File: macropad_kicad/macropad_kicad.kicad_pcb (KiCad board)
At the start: 2 copper layers, 26 parts, among them J1 OLED_128x64, SW1 RotaryEncoder_Switch, U1 MOUDLE-SEEEDUINO-XIAO

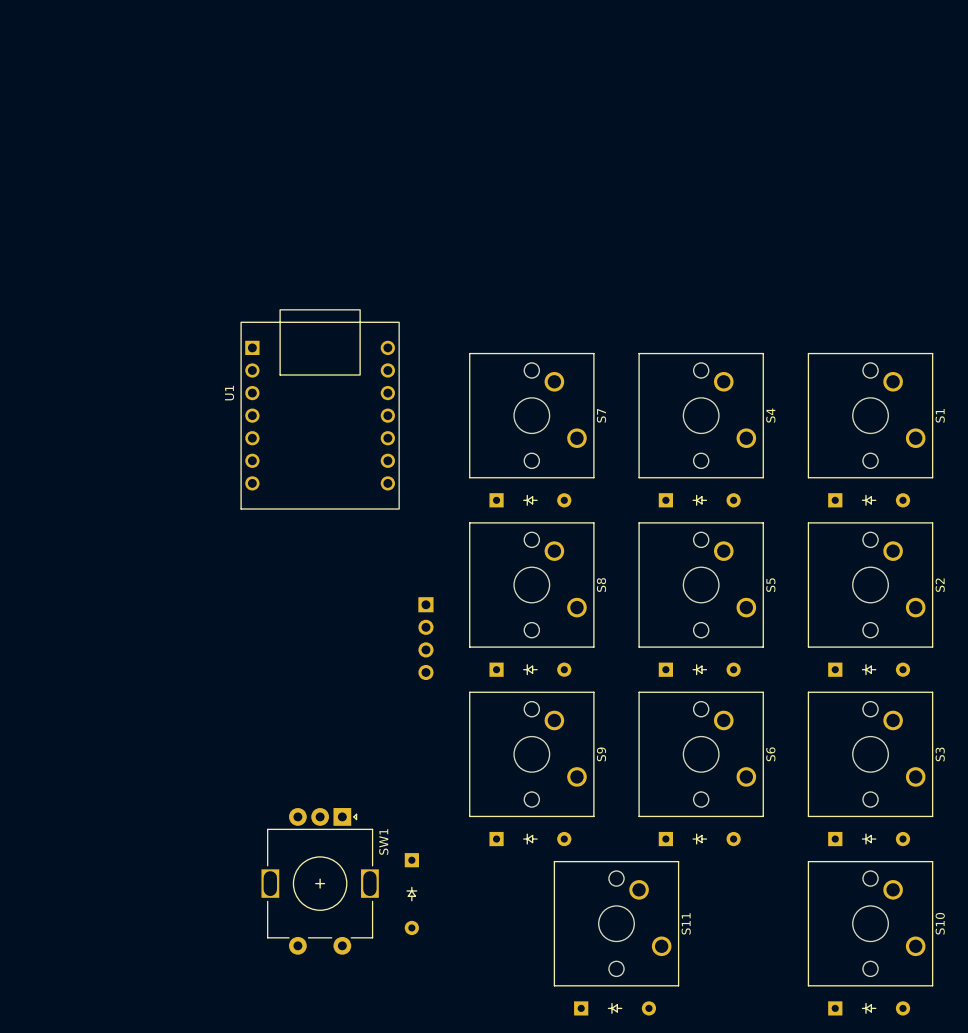
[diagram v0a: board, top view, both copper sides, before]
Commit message: fixed scheme
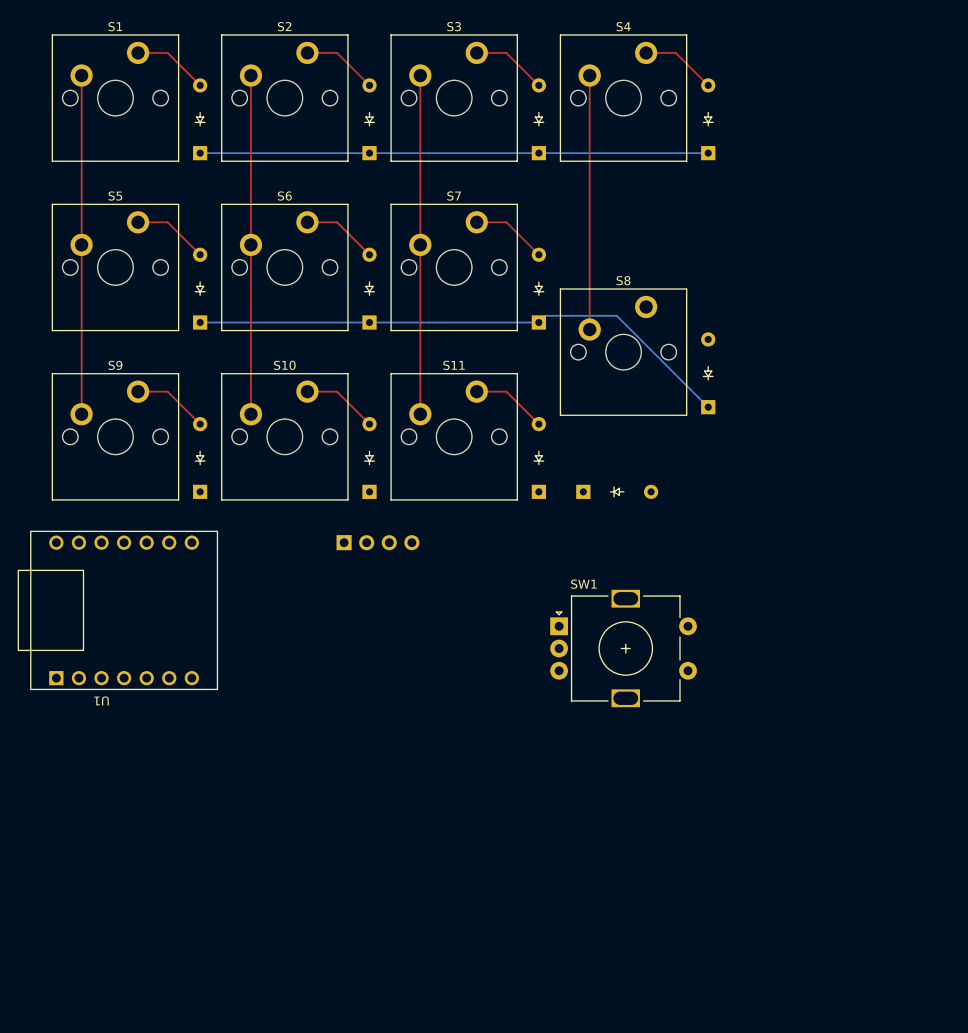
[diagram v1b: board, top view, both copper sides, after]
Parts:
- S1, S10, S11, S2, S3, S4, S5, S6, S7, S8, S9: footprint Button_Switch_Keyboard:SW_Cherry_MX_1.00u_PCB -> ScottoKeebs_MX:MX_PCB_1.00u
- moved S1 97.8 mm to (57.1, 38.1), turned to 0 degrees
- moved S3 92.3 mm to (95.2, 38.1), turned to 0 degrees
- moved S10 91.2 mm to (76.2, 76.2), turned to 0 degrees
- moved S2 91.2 mm to (76.2, 38.1), turned to 0 degrees
- moved D7 84.0 mm to (104.8, 63.3), turned to 90 degrees
- moved S5 80.6 mm to (57.1, 57.1), turned to 0 degrees
- moved D4 78.5 mm to (123.8, 44.3), turned to 90 degrees
- moved D5 78.2 mm to (66.7, 63.3), turned to 90 degrees
- moved S6 77.3 mm to (76.2, 57.1), turned to 0 degrees
- moved D8 69.1 mm to (123.8, 72.9), turned to 90 degrees
- moved D2 67.0 mm to (85.7, 44.3), turned to 90 degrees
- moved D3 67.0 mm to (104.8, 44.3), turned to 90 degrees
- moved D1 65.3 mm to (66.7, 44.3), turned to 90 degrees
- moved S9 64.5 mm to (57.1, 76.2), turned to 0 degrees
- moved S11 61.9 mm to (95.2, 76.2), turned to 0 degrees
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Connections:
- D1 pad 1: (no net) -> Row 0
- D1 pad 2: (no net) -> Net-(D1-A)
- D10 pad 1: Row 0 -> Row 2
- D10 pad 2: (no net) -> Net-(D10-A)
- D11 pad 1: Row 1 -> Row 2
- D11 pad 2: (no net) -> Net-(D11-A)
- D12 pad 2: (no net) -> Net-(D12-A)
- D2 pad 2: (no net) -> Net-(D2-A)
- D3 pad 2: (no net) -> Net-(D3-A)
- D4 pad 1: (no net) -> Row 0
- D4 pad 2: (no net) -> Net-(D4-A)
- D5 pad 2: (no net) -> Net-(D5-A)
- D6 pad 2: (no net) -> Net-(D6-A)
- D7 pad 1: (no net) -> Row 1
- D7 pad 2: (no net) -> Net-(D7-A)
- D8 pad 1: Row 2 -> Row 1
- D8 pad 2: (no net) -> Net-(D8-A)
- D9 pad 2: (no net) -> Net-(D9-A)
- J1 pad 1: (no net) -> GND
- J1 pad 2: (no net) -> +5V
- J1 pad 3: (no net) -> SCL
- J1 pad 4: (no net) -> SDA
- S1 pad 1: (no net) -> Col 0
- S1 pad 2: Net-(D3-A) -> Net-(D1-A)
- S10 pad 1: (no net) -> Col 1
- S11 pad 1: Col 3 -> Col 2
- S2 pad 1: (no net) -> Col 1
- S2 pad 2: Net-(D1-A) -> Net-(D2-A)
- S3 pad 1: (no net) -> Col 2
- S3 pad 2: Net-(D2-A) -> Net-(D3-A)
- S4 pad 1: Col 0 -> Col 3
- S5 pad 1: Col 1 -> Col 0
- S6 pad 1: Col 2 -> Col 1
- S7 pad 1: Col 0 -> Col 2
- S8 pad 1: Col 1 -> Col 3
- S9 pad 1: Col 2 -> Col 0
- SW1 pad A: (no net) -> Rot A
- SW1 pad B: (no net) -> Rot B
- U1 pad 12: (no net) -> +3.3V
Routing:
- net Row 1: track 0.00 -> 61.7 mm
- net Row 0: track 0.00 -> 57.2 mm
- net Col 2: track 0.00 -> 38.1 mm
- net Col 1: track 0.00 -> 38.1 mm
- net Col 0: track 0.00 -> 38.1 mm
- net Col 3: track 0.00 -> 28.6 mm
- net Net-(D6-A): track 0.00 -> 8.50 mm
- net Net-(D2-A): track 0.00 -> 8.50 mm
- net Net-(D5-A): track 0.00 -> 8.50 mm
- net Net-(D1-A): track 0.00 -> 8.50 mm
- net Net-(D7-A): track 0.00 -> 8.50 mm
- net Net-(D4-A): track 0.00 -> 8.50 mm
- net Net-(D3-A): track 0.00 -> 8.50 mm
- net Net-(D10-A): track 0.00 -> 8.50 mm
- net Net-(D9-A): track 0.00 -> 8.50 mm
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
